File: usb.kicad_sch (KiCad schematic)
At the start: 63 parts, among them J13 USB-C_GCT_USB4105-GF-A, J3 USB-C_GCT_USB4105-GF-A, Q1 SSM3J332R, Q2 BC817-25W, Q3 BCM857BS-7-F, Q4 SSM3J332R, Q5 BCM857BS-7-F, U11 AP22652W6, U15 AP22652W6, U2 TPD4E05U06QDQARQ1, U4 AP62301_TSOT, U5 TPD4E05U06QDQARQ1, U8 AP62301_TSOT

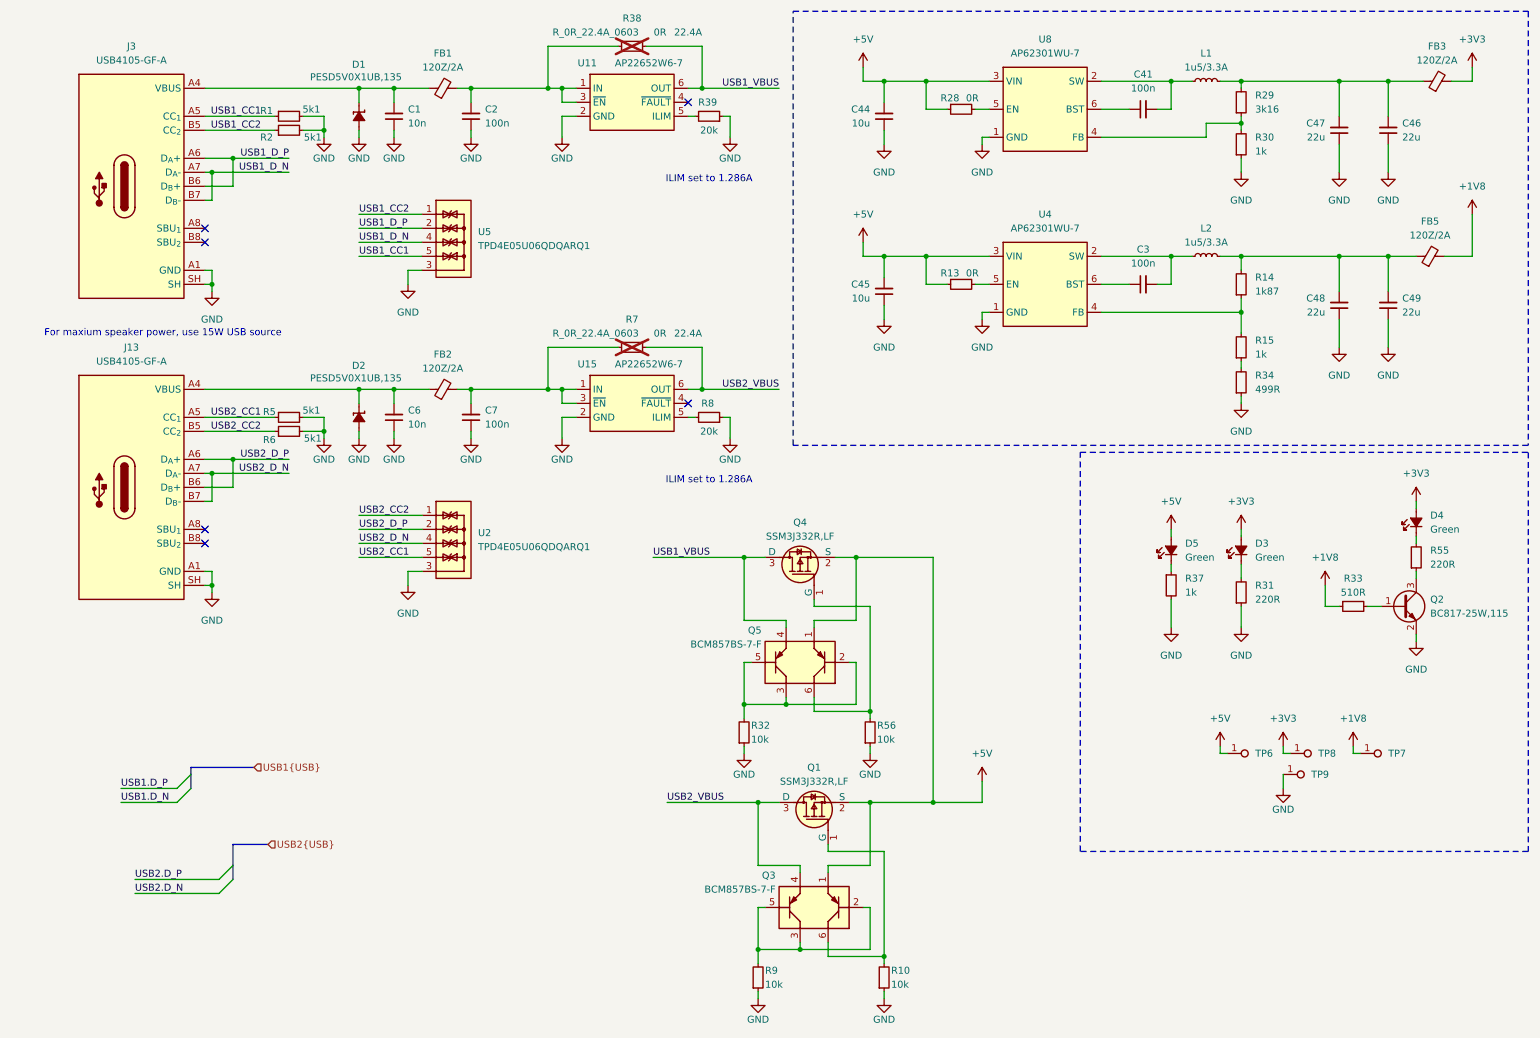
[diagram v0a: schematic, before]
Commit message: [#71555] Draw MIC and USB Connector sheets
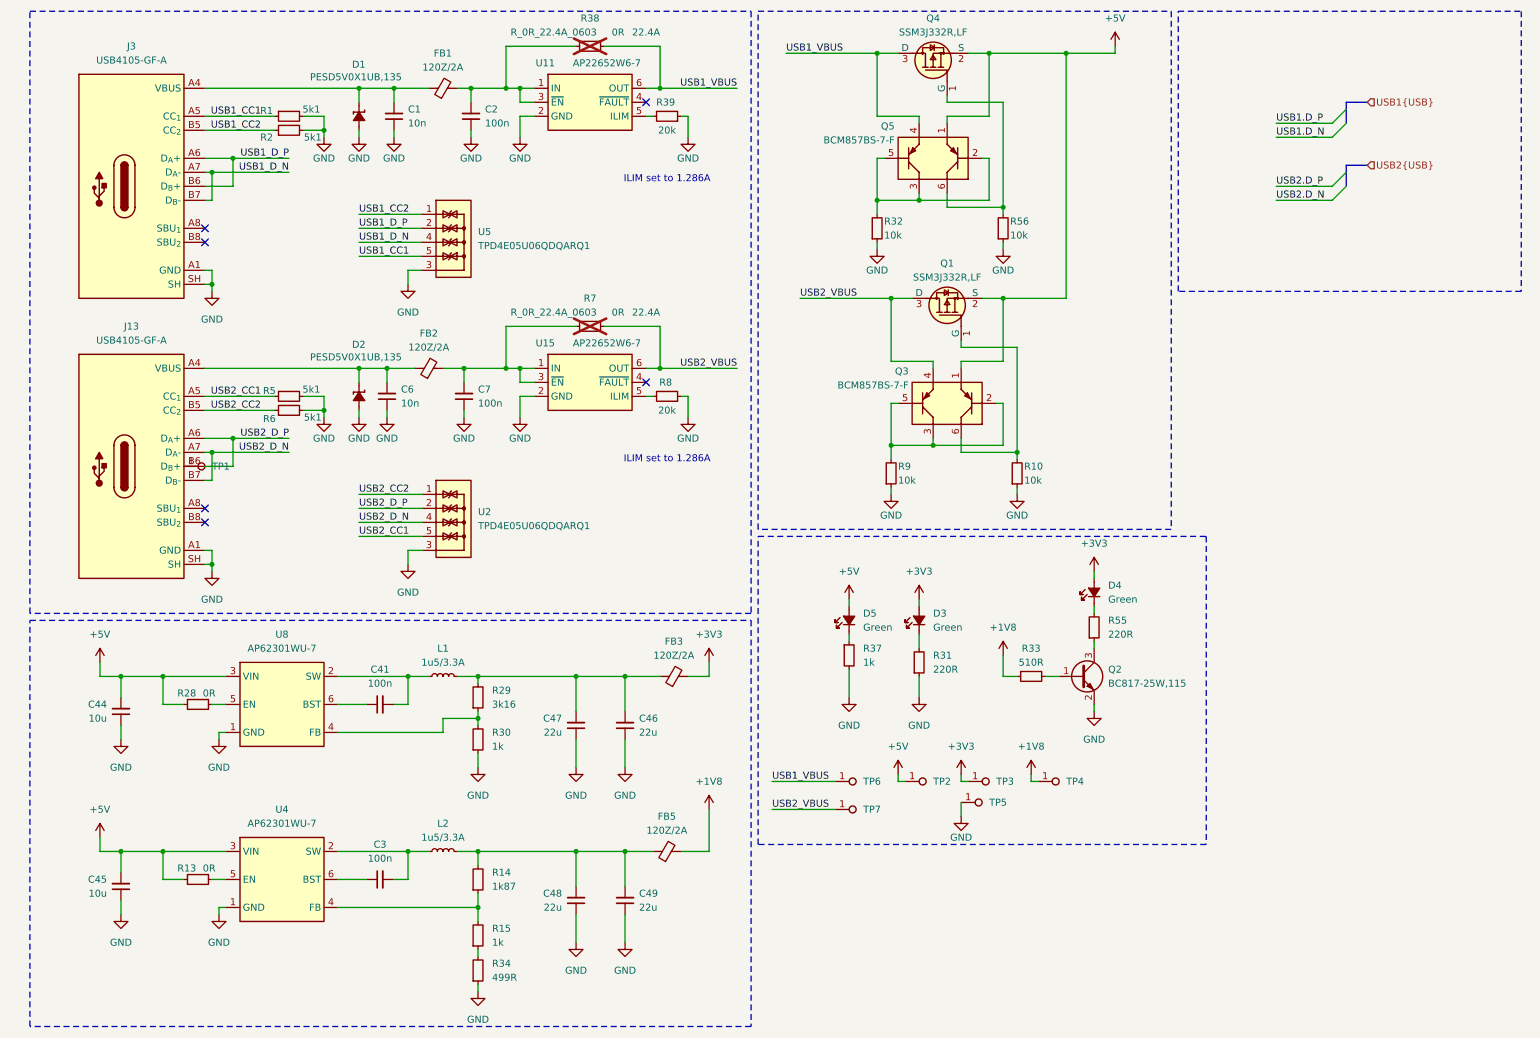
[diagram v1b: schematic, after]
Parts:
- removed TP6, TP7, TP8, TP9: TP_1.5mm_SMD, antmicro-footprints:TP_SMD_1.5mm, symbol antmicroTestPoints:TP_1.5mm_SMD
- added TP1, TP2, TP3, TP4, TP5, TP6, TP7: TP_0.75mm_SMD, antmicro-footprints:TP_SMD_0.75mm, symbol antmicroTestPoints:TP_0.75mm_SMD
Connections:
- net +1V8: now also TP4.1
- net +3V3: now also TP3.1
- net +5V: now also TP2.1
- net GND: now also TP5.1
- net USB1_VBUS: now also TP6.1
- net USB2_VBUS: now also TP7.1
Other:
- note removed: "For maxium speaker power, use 15W USB source"
- moved on the sheet: C3, C41, C44, C45, C46, C47, C48, C49, C6, C7, D2, D3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
